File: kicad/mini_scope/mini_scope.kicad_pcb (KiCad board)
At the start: 2 copper layers, 67.5 x 60 mm, 65 parts, among them J1 USB_B_Mini, J2 Conn_Coaxial, J3 Conn_01x03_Male, J4 STK3700_exp_conn, K1 G5LE-1, Q1 BC848, U1 FT232RL, U2 OPA340UA, U3 OPA340UA, U4 TLP2761, U5 TLP2761, U6 CRE1S0505SC

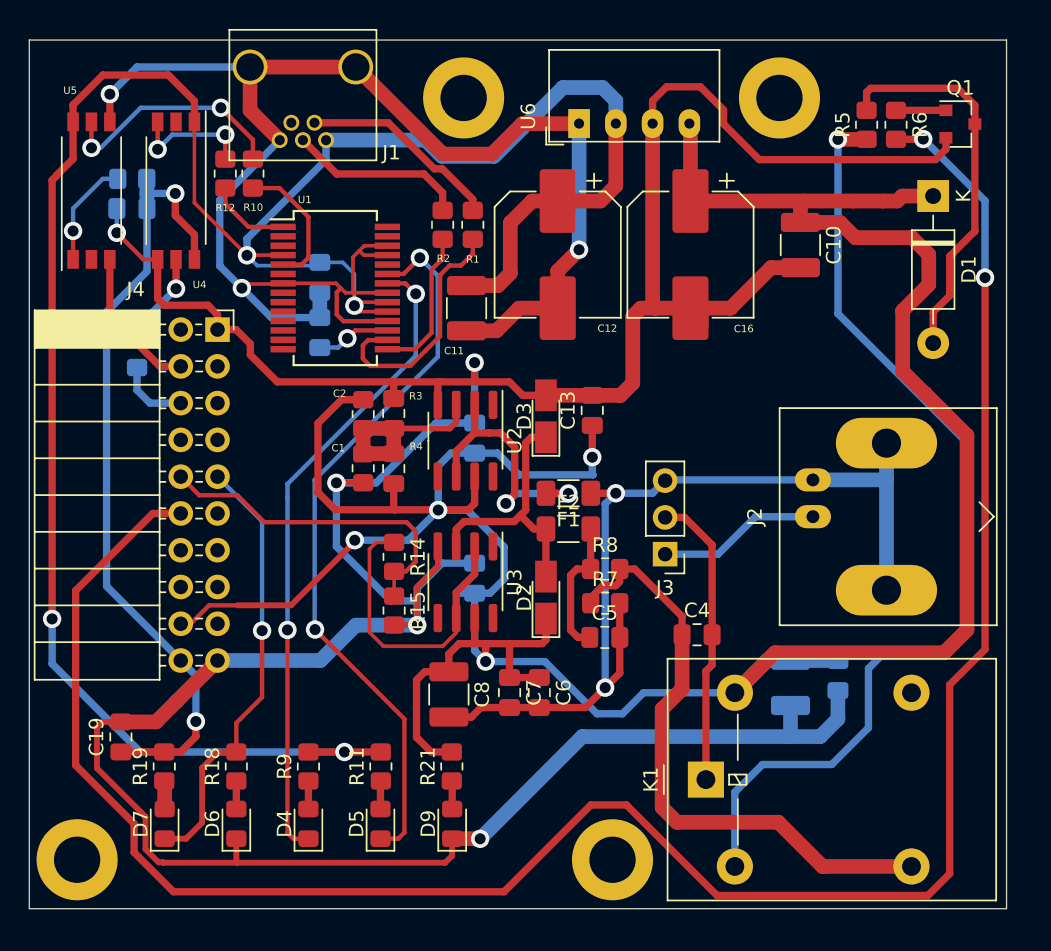
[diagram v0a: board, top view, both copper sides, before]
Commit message: project refresh
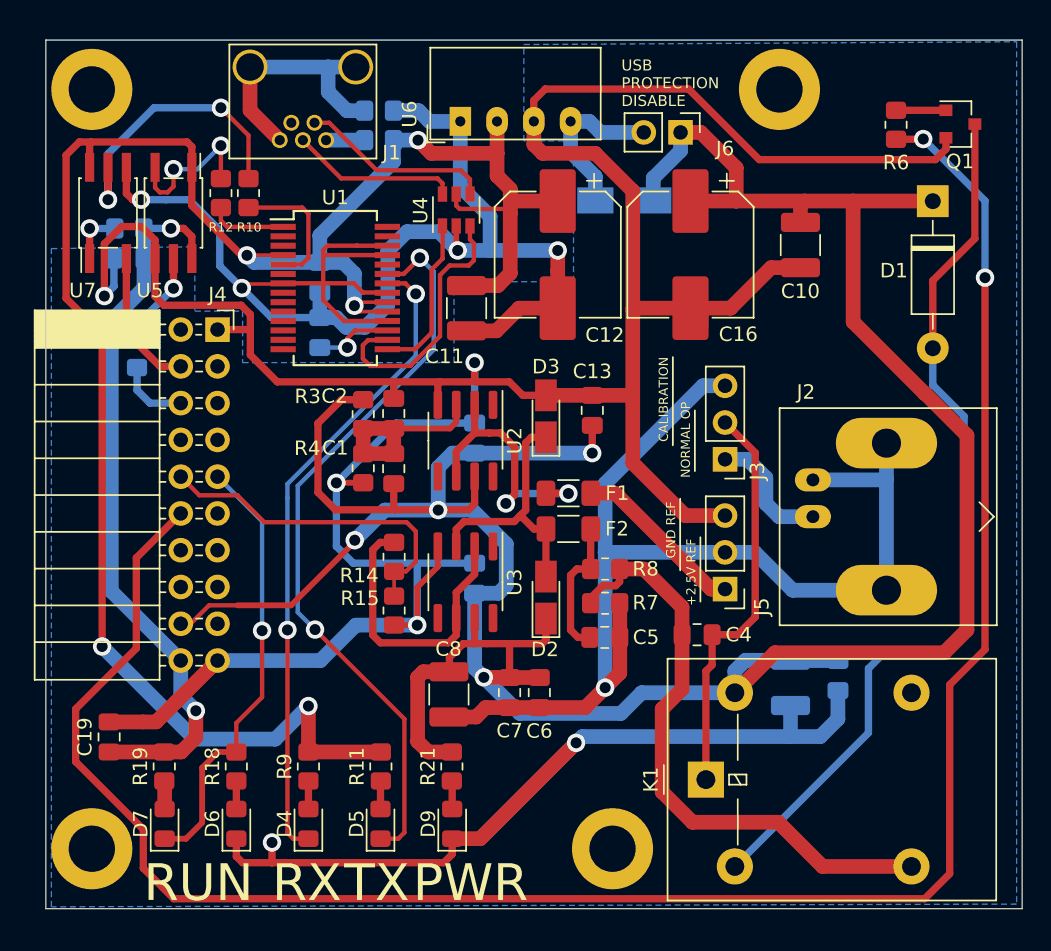
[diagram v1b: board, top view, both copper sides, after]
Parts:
- removed R1, R2: 22, Resistor_SMD:R_0805_2012Metric_Pad1.20x1.40mm_HandSolder
- removed R5: 1k, Resistor_SMD:R_0805_2012Metric_Pad1.20x1.40mm_HandSolder
- added D8: D_Schottky, Diode_SMD:D_SMA, B.Cu at (58.1, 71.1)
- added FB1: Ferrite_Bead_Small, Resistor_SMD:R_0805_2012Metric_Pad1.20x1.40mm_HandSolder, B.Cu at (41.2, 66.9)
- added FB2: Ferrite_Bead_Small, Resistor_SMD:R_0805_2012Metric_Pad1.20x1.40mm_HandSolder, B.Cu at (41.2, 64.9)
- added G***: LOGO, mini_scope:logo, B.Cu at (45.3, 108.3)
- added J5: Conn_01x03_Male, Connector_PinHeader_2.54mm:PinHeader_1x03_P2.54mm_Vertical, F.Cu at (65.1, 97.9)
- added J6: Conn_01x02_Male, Connector_PinHeader_2.54mm:PinHeader_1x02_P2.54mm_Vertical, F.Cu at (62.0, 66.4)
- added U7: TLP2368, Package_SO:SO-5_4.4x3.6mm_P1.27mm, F.Cu at (22.4, 71.9)
- U1: footprint Package_SO:SSOP-28_5.3x10.2mm_P0.65mm -> mini_scope:SSOP-28_5.3x10.2mm_P0.65mm
- U4: value TLP2761 -> USBLC6-2SC6; footprint Package_SO:SO-6L_10x3.84mm_P1.27mm -> Package_TO_SOT_SMD:SOT-23-6
- U5: value TLP2761 -> TLP2368; footprint Package_SO:SO-6L_10x3.84mm_P1.27mm -> Package_SO:SO-5_4.4x3.6mm_P1.27mm
- moved H3 25.7 mm to (21.3, 63.4)
- moved U4 19.4 mm to (46.5, 71.7), turned to 90 degrees
- moved U6 8.21 mm to (46.8, 65.6)
- moved J3 7.75 mm to (65.1, 89.0)
- moved U5 5.87 mm to (27.0, 71.9), turned to 270 degrees
- moved C17 3.44 mm to (23.9, 75.1)
- moved R16 3.44 mm to (23.9, 73.0)
- moved R10 1.38 mm to (32.1, 70.6)
- moved R12 1.38 mm to (30.2, 70.6)
- moved H1 1.27 mm to (21.3, 115.9)
- moved C19 0.81 mm to (22.5, 108.1)
- moved H2 0.76 mm to (57.3, 115.9)
- moved H4 0.59 mm to (68.8, 63.4)
- moved D1 0.36 mm to (79.4, 71.1)
- turned C3 to 270 degrees
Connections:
- C3 pad 1: Net-(C3-Pad1) -> Earth
- C3 pad 2: Earth -> Net-(C3-Pad2)
- F1 pad 1: GNDREF -> Net-(F1-Pad1)
- J1 pad 1: VBUS -> Net-(FB1-Pad1)
- J1 pad 5: Earth -> Net-(FB2-Pad2)
- J1 pad 6: Earth -> Net-(FB2-Pad2)
- J1 pad 7: Earth -> Net-(FB2-Pad2)
- K1 pad 2: Net-(K1-Pad2) -> Net-(D1-Pad2)
- U1 pad 15: Net-(R2-Pad2) -> Net-(U1-Pad15)
- U1 pad 16: Net-(R1-Pad2) -> Net-(U1-Pad16)
- U1 pad 17: Net-(C3-Pad1) -> Net-(C3-Pad2)
- U4 pad 1: VBUS -> Net-(U1-Pad15)
- U4 pad 2: Net-(U4-Pad2) -> Earth
- U4 pad 3: Net-(R12-Pad1) -> Net-(U1-Pad16)
- U4 pad 4: GND -> Net-(J1-Pad2)
- U4 pad 5: Net-(R17-Pad1) -> VBUS
- U4 pad 6: +3V3 -> Net-(J1-Pad3)
- U5 pad 1: Net-(R16-Pad2) -> VBUS
- U5 pad 3: TX -> Net-(R12-Pad1)
- U5 pad 4: Earth -> GND
- U5 pad 5: Net-(R10-Pad1) -> Net-(R17-Pad1)
- U5 pad 6: VBUS -> +3V3
- U6 pad 4: +5V -> Net-(D8-Pad2)
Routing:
- net Net-(K1-Pad2): track 67.6 -> 0.00 mm, vias 1 -> 0
- net Net-(D1-Pad2): track 26.9 -> 62.3 mm
- net GND: track 247.2 -> 276.2 mm, vias 5 -> 6
- net VBUS: track 160.8 -> 139.5 mm, vias 4 -> 5
- net Net-(U1-Pad16): track 0.00 -> 18.6 mm
- net Net-(FB2-Pad2): track 0.00 -> 18.0 mm
- net Net-(R1-Pad2): track 17.3 -> 0.00 mm
- net GNDREF: track 62.7 -> 78.9 mm, vias 2 -> 1
- net Net-(F1-Pad1): track 0.00 -> 12.0 mm
- net Net-(D8-Pad2): track 0.00 -> 11.5 mm
- net Net-(U1-Pad15): track 0.00 -> 11.2 mm
- net Net-(R2-Pad2): track 10.3 -> 0.00 mm
- net Earth: track 108.5 -> 99.6 mm, vias 3 -> 4
- net Net-(C4-Pad2): track 20.4 -> 28.0 mm
- net ac_dc_couple: track 147.8 -> 142.2 mm
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- added copper zone on B.Cu, net GND
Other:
- board size 67.5 x 60 mm -> 67.4 x 60 mm
- board text added: "+2,5V REF"
- board text added: "CALIBRATION"
- board text added: "CONFIG JUMPERS: J3: SELECT CALIBRATION / MEASURE MODE J5: SELECT GROUND REFERENCE J6: DISABLE POWER PROTECTION DIODE"
- board text added: "GND REF"
- board text added: "MiniScope V100 Designed by Mihaly Szabo"
- board text added: "NORMAL OP"
- board text added: "PWR"
- board text added: "RUN"
- board text added: "RX"
- board text added: "TX"
- board text added: "USB PROTECTION DISABLE"
